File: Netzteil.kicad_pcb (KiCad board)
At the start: 2 copper layers, 61 x 27 mm, 15 parts, among them J1 Conn_01x02_Socket, J2 Conn_01x02_Socket, J3 J-jumper, P1 P-trim, U1 LM2596S-ADJ

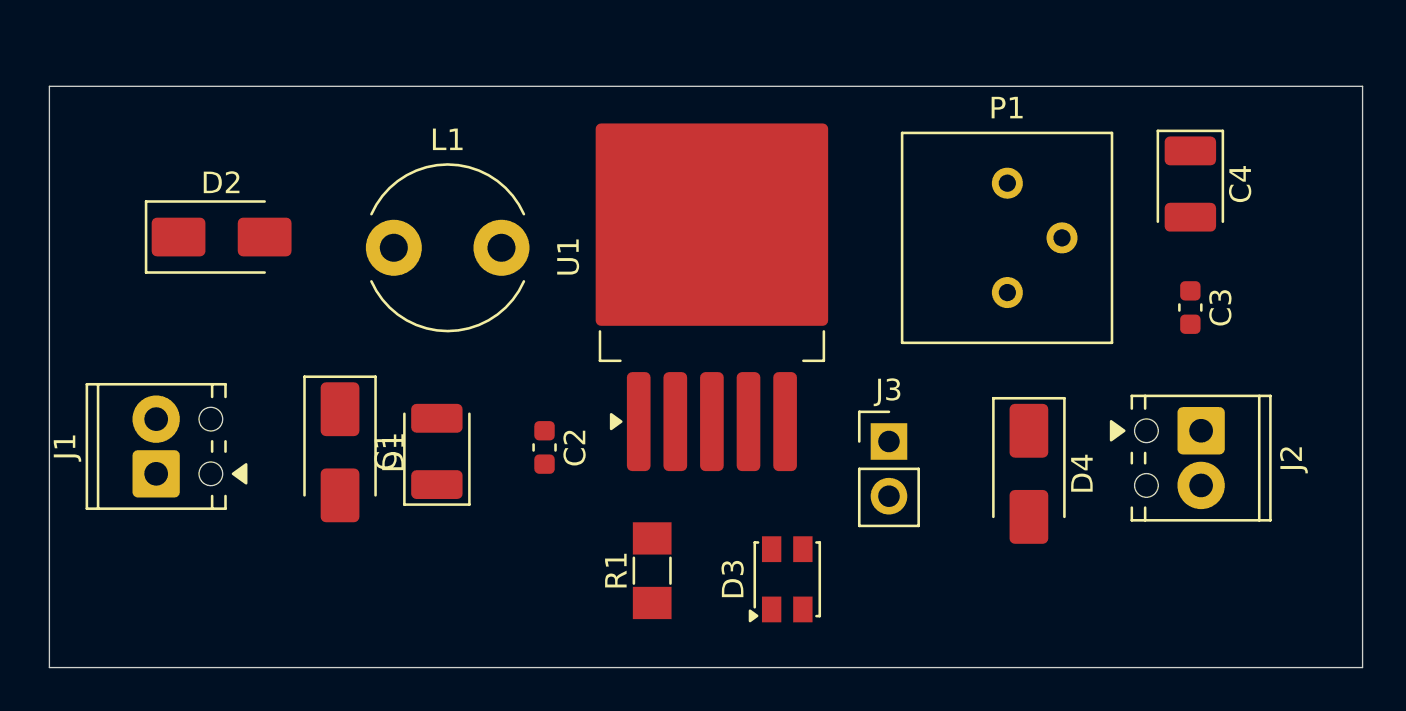
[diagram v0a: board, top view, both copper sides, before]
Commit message: First Routes.
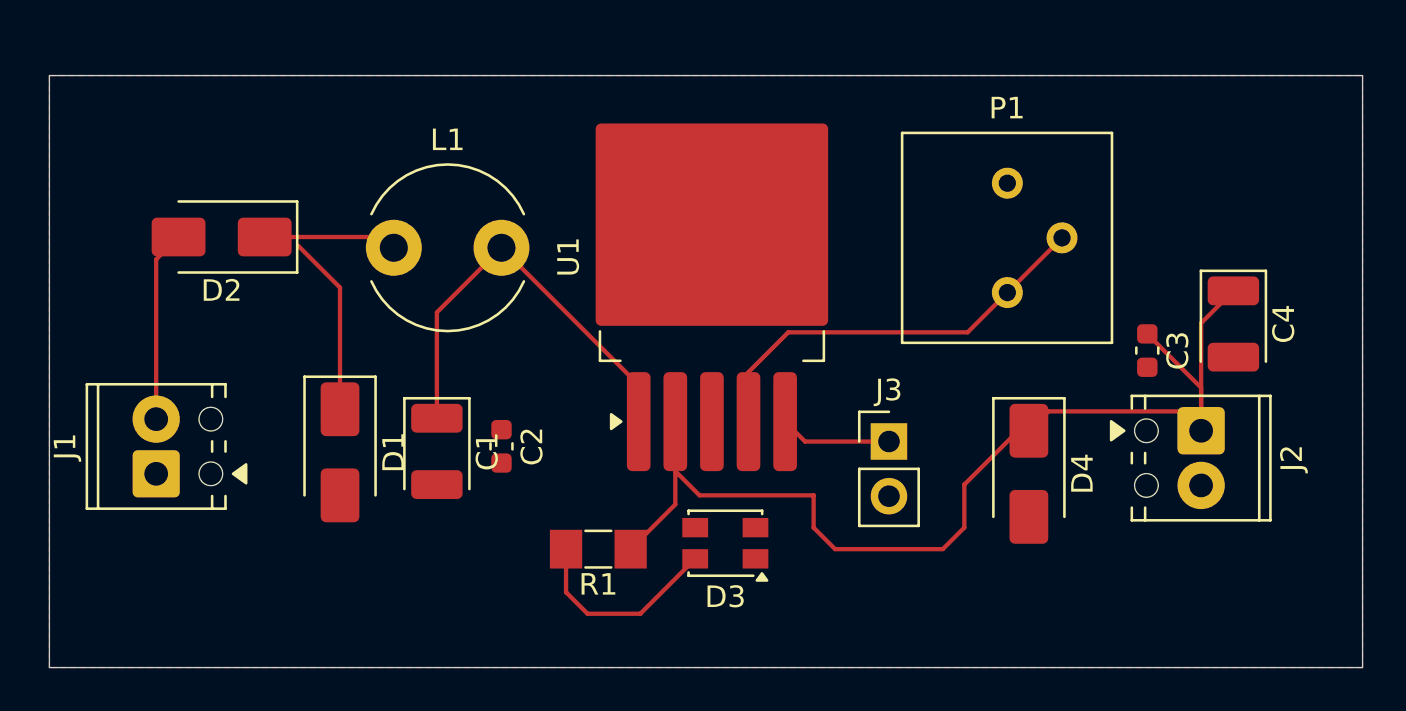
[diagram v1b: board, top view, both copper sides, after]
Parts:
- moved C4 6.80 mm to (171.5, 59.0)
- moved D3 3.33 mm to (147.9, 69.2), turned to 180 degrees
- moved C3 2.83 mm to (167.5, 60.3)
- moved R1 2.69 mm to (142.0, 69.5), turned to 180 degrees
- moved C2 2.00 mm to (137.5, 64.7)
- turned C1 to -90 degrees
- turned D2 to 180 degrees
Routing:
- net Net-(C3-+): track 0.00 -> 52.7 mm
- net Net-(C1-+): track 0.00 -> 19.9 mm
- net Net-(P1-a): track 0.00 -> 19.4 mm
- net +VDC: track 0.00 -> 17.3 mm
- net Net-(D3-A): track 0.00 -> 9.47 mm
- net Net-(C2-+): track 0.00 -> 6.21 mm
- net Net-(U1-~{ON}/OFF): track 0.00 -> 5.92 mm
- added copper zone on F.Cu, net V-GND
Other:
- board size 61 x 27 mm -> 61 x 27.5 mm

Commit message: Second try routing.
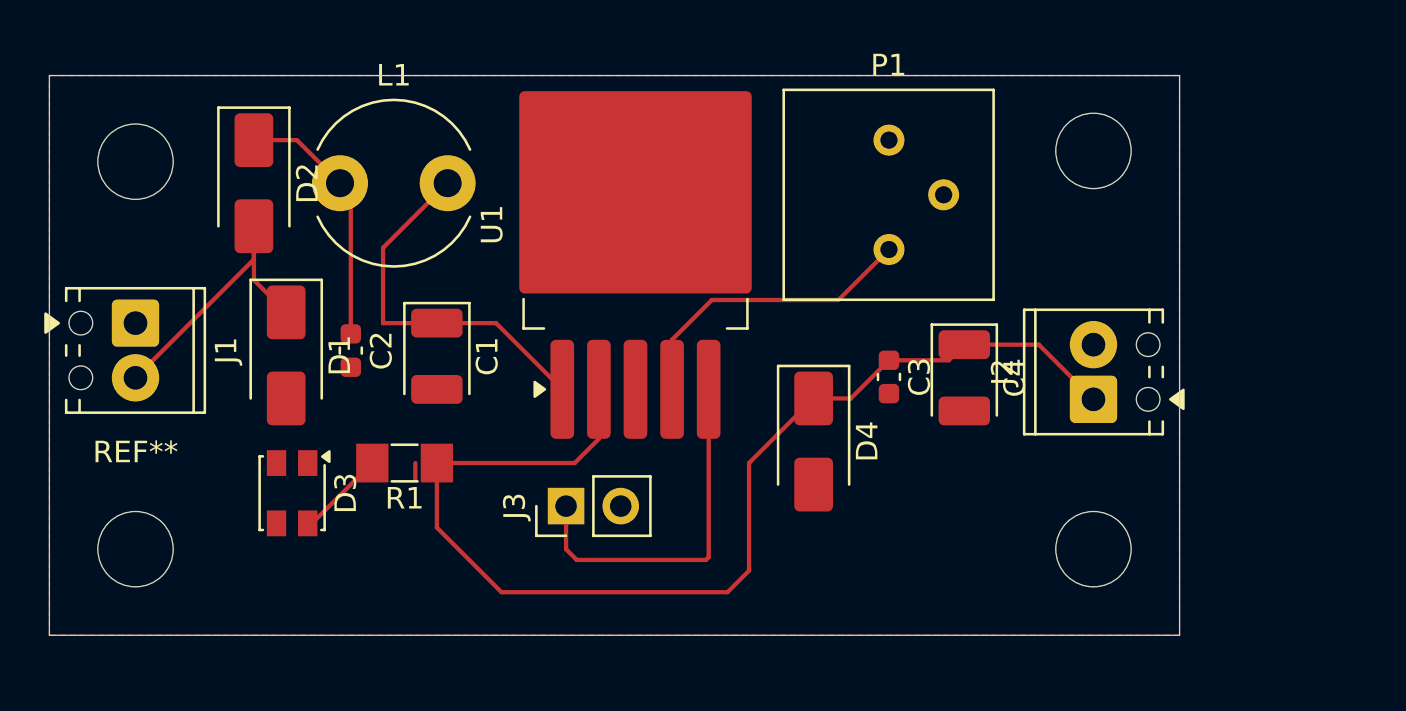
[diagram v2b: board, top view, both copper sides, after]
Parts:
- added REF**: MountingHole_3.5mm, MountingHole:MountingHole_3.5mm, F.Cu at (165.0, 51.0)
- added REF**: MountingHole_3.5mm, MountingHole:MountingHole_3.5mm, F.Cu at (120.5, 69.5)
- added REF**: MountingHole_3.5mm, MountingHole:MountingHole_3.5mm, F.Cu at (120.5, 51.5)
- added REF**: MountingHole_3.5mm, MountingHole:MountingHole_3.5mm, F.Cu at (165.0, 69.5)
- moved D3 20.3 mm to (127.8, 66.9), turned to -90 degrees
- moved J3 15.3 mm to (140.5, 67.5), turned to 90 degrees
- moved C4 12.7 mm to (159.0, 61.5)
- moved C3 12.1 mm to (155.5, 61.5)
- moved D4 10.1 mm to (152.0, 64.5)
- moved R1 9.85 mm to (133.0, 65.5)
- moved C2 8.29 mm to (130.5, 60.3)
- moved J1 7.07 mm to (120.5, 59.0), turned to -90 degrees
- moved P1 5.85 mm to (155.5, 55.6)
- moved J2 5.21 mm to (165.0, 62.5), turned to 90 degrees
- moved D1 5.15 mm to (127.5, 60.5)
- moved C1 4.42 mm to (134.5, 60.5)
- moved L1 3.91 mm to (130.0, 52.5)
- moved U1 3.85 mm to (143.7, 54.4)
- moved D2 2.92 mm to (126.0, 52.5), turned to -90 degrees
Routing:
- net Net-(U1-~{ON}/OFF): track 5.92 -> 16.7 mm
- net Net-(C2-+): track 6.21 -> 12.0 mm
- net Net-(P1-a): track 19.4 -> 14.1 mm
- net Net-(D3-A): track 9.47 -> 4.91 mm
- net +VDC: track 17.3 -> 13.9 mm
- net Net-(C1-+): track 19.9 -> 17.3 mm
- net Net-(C3-+): track 52.7 -> 53.8 mm
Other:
- board size 61 x 27.5 mm -> 52.5 x 26 mm
